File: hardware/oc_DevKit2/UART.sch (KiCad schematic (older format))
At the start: 6 parts, among them U1 CP2102N

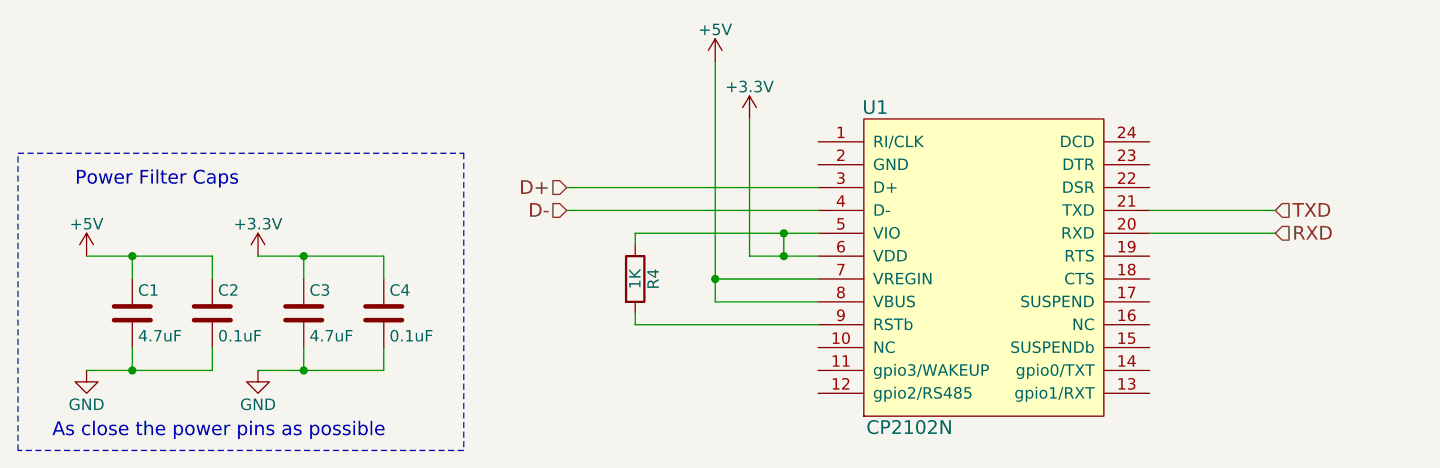
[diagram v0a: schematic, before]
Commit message: Lil Patch
Small changes. Updating for forthcoming Lite branch updates
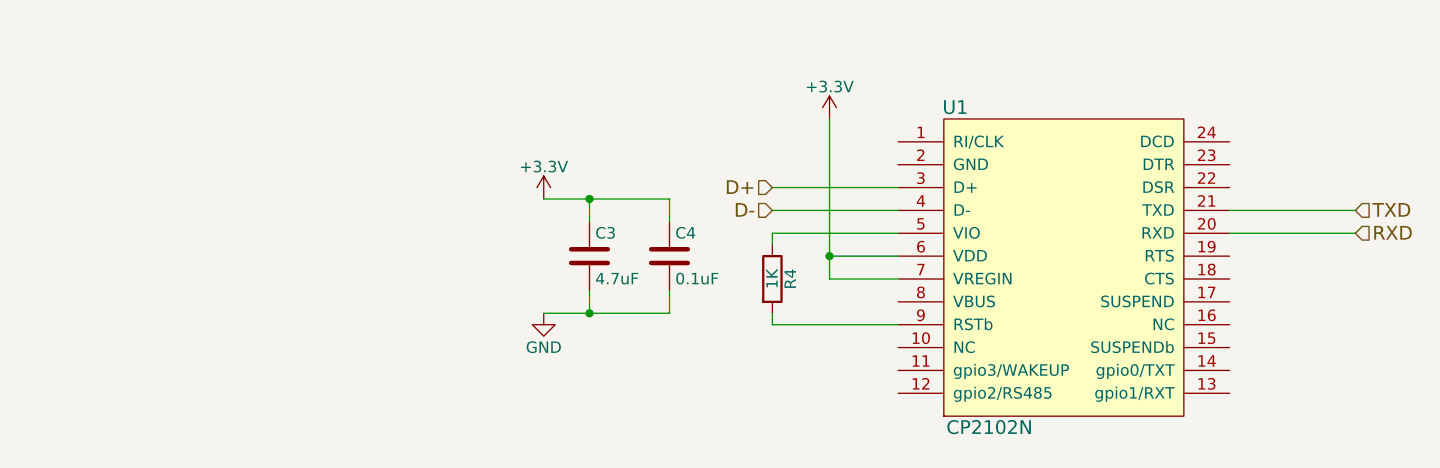
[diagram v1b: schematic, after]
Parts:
- removed C1: 4.7uF, Capacitors_SMD:C_0805_HandSoldering, symbol C
- removed C2: 0.1uF, Capacitors_SMD:C_0805_HandSoldering, symbol C
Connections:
- net +3V3: now also U1.7 (VREGIN); no longer R4.1, U1.5 (VIO)
- net +5V: no longer names the net of U1.8 (VBUS)
- net +5V: no longer U1.7 (VREGIN)
- new net: R4.1, U1.5 (VIO)
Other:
- note removed: "As close the power pins as possible"
- note removed: "Power Filter Caps"
- moved on the sheet: C3, C4, R4, U1
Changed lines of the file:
@@
 L CP2102N U1
 U 1 1 59C93D7F
-P 5850 4600
-F 0 "U1" H 5350 5950 60  0000 C CNN
-F 1 "CP2102N" H 5500 4550 60  0000 C CNN
-F 2 "Housings_DFN_QFN:QFN-24_4x4mm_Pitch0.5mm" H 5700 4600 60  0001 C CNN
-F 3 "" H 5700 4600 60  0001 C CNN
-	1    5850 4600
+P 6200 4600
+F 0 "U1" H 5700 5950 60  0000 C CNN
+F 1 "CP2102N" H 5850 4550 60  0000 C CNN
+F 2 "Housings_DFN_QFN:QFN-24_4x4mm_Pitch0.5mm" H 6050 4600 60  0001 C CNN
+F 3 "" H 6050 4600 60  0001 C CNN
+	1    6200 4600
 	1    0    0    -1
 $EndComp
@@
 L R R4
 U 1 1 59C9487D
-P 4300 4000
-F 0 "R4" V 4380 4000 50  0000 C CNN
-F 1 "1K" V 4300 4000 50  0000 C CNN
-F 2 "Resistors_SMD:R_0805_HandSoldering" V 4230 4000 50  0001 C CNN
-F 3 "" H 4300 4000 50  0001 C CNN
-	1    4300 4000
+P 4900 4000
+F 0 "R4" V 4980 4000 50  0000 C CNN
+F 1 "1K" V 4900 4000 50  0000 C CNN
+F 2 "Resistors_SMD:R_0805_HandSoldering" V 4830 4000 50  0001 C CNN
+F 3 "" H 4900 4000 50  0001 C CNN
+	1    4900 4000
 	1    0    0    -1
 $EndComp
@@
 L C C3
 U 1 1 59C94915
-P 2850 4150
-F 0 "C3" H 2875 4250 50  0000 L CNN
-F 1 "4.7uF" H 2875 4050 50  0000 L CNN
-F 2 "Capacitors_SMD:C_0805_HandSoldering" H 2888 4000 50  0001 C CNN
-F 3 "" H 2850 4150 50  0001 C CNN
-	1    2850 4150
-	1    0    0    -1
-$EndComp
-$Comp
-L C C1
-U 1 1 59C94A49
-P 2100 4150
-F 0 "C1" H 2125 4250 50  0000 L CNN
-F 1 "4.7uF" H 2125 4050 50  0000 L CNN
-F 2 "Capacitors_SMD:C_0805_HandSoldering" H 2138 4000 50  0001 C CNN
-F 3 "" H 2100 4150 50  0001 C CNN
-	1    2100 4150
-	1    0    0    -1
-$EndComp
-$Comp
-L C C2
-U 1 1 59C94A6F
-P 2450 4150
-F 0 "C2" H 2475 4250 50  0000 L CNN
-F 1 "0.1uF" H 2475 4050 50  0000 L CNN
-F 2 "Capacitors_SMD:C_0805_HandSoldering" H 2488 4000 50  0001 C CNN
-F 3 "" H 2450 4150 50  0001 C CNN
-	1    2450 4150
+P 4100 3900
+F 0 "C3" H 4125 4000 50  0000 L CNN
+F 1 "4.7uF" H 4125 3800 50  0000 L CNN
+F 2 "Capacitors_SMD:C_0805_HandSoldering" H 4138 3750 50  0001 C CNN
+F 3 "" H 4100 3900 50  0001 C CNN
+	1    4100 3900
 	1    0    0    -1
 $EndComp
@@
 L C C4
 U 1 1 59C94ADB
-P 3200 4150
-F 0 "C4" H 3225 4250 50  0000 L CNN
-F 1 "0.1uF" H 3225 4050 50  0000 L CNN
-F 2 "Capacitors_SMD:C_0805_HandSoldering" H 3238 4000 50  0001 C CNN
-F 3 "" H 3200 4150 50  0001 C CNN
-	1    3200 4150
+P 4450 3900
+F 0 "C4" H 4475 4000 50  0000 L CNN
+F 1 "0.1uF" H 4475 3800 50  0000 L CNN
+F 2 "Capacitors_SMD:C_0805_HandSoldering" H 4488 3750 50  0001 C CNN
+F 3 "" H 4450 3900 50  0001 C CNN
+	1    4450 3900
 	1    0    0    -1
 $EndComp
@@
 L GND #PWR017
 U 1 1 59C94DA8
-P 2650 4400
-F 0 "#PWR017" H 2650 4150 50  0001 C CNN
-F 1 "GND" H 2650 4250 50  0000 C CNN
-F 2 "" H 2650 4400 50  0001 C CNN
-F 3 "" H 2650 4400 50  0001 C CNN
-	1    2650 4400
+P 3900 4150
+F 0 "#PWR017" H 3900 3900 50  0001 C CNN
+F 1 "GND" H 3900 4000 50  0000 C CNN
+F 2 "" H 3900 4150 50  0001 C CNN
+F 3 "" H 3900 4150 50  0001 C CNN
+	1    3900 4150
 	1    0    0    -1
 $EndComp
 $Comp
-L GND #PWR018
-U 1 1 59C94DCF
-P 1900 4400
-F 0 "#PWR018" H 1900 4150 50  0001 C CNN
-F 1 "GND" H 1900 4250 50  0000 C CNN
-F 2 "" H 1900 4400 50  0001 C CNN
-F 3 "" H 1900 4400 50  0001 C CNN
-	1    1900 4400
+L +3.3V #PWR018
+U 1 1 59C94E0C
+P 3900 3650
+F 0 "#PWR018" H 3900 3500 50  0001 C CNN
+F 1 "+3.3V" H 3900 3790 50  0000 C CNN
+F 2 "" H 3900 3650 50  0001 C CNN
+F 3 "" H 3900 3650 50  0001 C CNN
+	1    3900 3650
 	1    0    0    -1
 $EndComp
 $Comp
-L +5V #PWR019
-U 1 1 59C94DEA
-P 1900 3900
-F 0 "#PWR019" H 1900 3750 50  0001 C CNN
-F 1 "+5V" H 1900 4040 50  0000 C CNN
-F 2 "" H 1900 3900 50  0001 C CNN
-F 3 "" H 1900 3900 50  0001 C CNN
-	1    1900 3900
-	1    0    0    -1
-$EndComp
-$Comp
-L +3.3V #PWR020
-U 1 1 59C94E0C
-P 2650 3900
-F 0 "#PWR020" H 2650 3750 50  0001 C CNN
-F 1 "+3.3V" H 2650 4040 50  0000 C CNN
-F 2 "" H 2650 3900 50  0001 C CNN
-F 3 "" H 2650 3900 50  0001 C CNN
-	1    2650 3900
-	1    0    0    -1
-$EndComp
-$Comp
-L +3.3V #PWR021
+L +3.3V #PWR019
 U 1 1 59C94E58
-P 4800 3300
-F 0 "#PWR021" H 4800 3150 50  0001 C CNN
-F 1 "+3.3V" H 4800 3440 50  0000 C CNN
-F 2 "" H 4800 3300 50  0001 C CNN
-F 3 "" H 4800 3300 50  0001 C CNN
-	1    4800 3300
-	1    0    0    -1
-$EndComp
-$Comp
-L +5V #PWR022
-U 1 1 59C94E99
-P 4650 3050
-F 0 "#PWR022" H 4650 2900 50  0001 C CNN
-F 1 "+5V" H 4650 3190 50  0000 C CNN
-F 2 "" H 4650 3050 50  0001 C CNN
-F 3 "" H 4650 3050 50  0001 C CNN
-	1    4650 3050
+P 5150 3300
+F 0 "#PWR019" H 5150 3150 50  0001 C CNN
+F 1 "+3.3V" H 5150 3440 50  0000 C CNN
+F 2 "" H 5150 3300 50  0001 C CNN
+F 3 "" H 5150 3300 50  0001 C CNN
+	1    5150 3300
 	1    0    0    -1
 $EndComp
 Wire Wire Line
-	5100 3800 4300 3800
+	5450 3800 4900 3800
 Wire Wire Line
-	4300 3800 4300 3850
+	4900 3800 4900 3850
 Wire Wire Line
-	4300 4150 4300 4200
+	4900 4150 4900 4200
 Wire Wire Line
-	4300 4200 5100 4200
+	4900 4200 5450 4200
 Wire Wire Line
-	1900 3900 2450 3900
+	3900 3650 4450 3650
 Wire Wire Line
-	2450 3900 2450 4000
+	4450 3650 4450 3750
 Wire Wire Line
-	2100 4000 2100 3900
-Connection ~ 2100 3900
+	3900 4150 4450 4150
 Wire Wire Line
-	2450 4400 2450 4300
+	4450 4150 4450 4050
 Wire Wire Line
-	1900 4400 2450 4400
+	4100 4150 4100 4050
+Connection ~ 4100 4150
 Wire Wire Line
-	2100 4300 2100 4400
-Connection ~ 2100 4400
+	4100 3750 4100 3650
+Connection ~ 4100 3650
 Wire Wire Line
-	2650 3900 3200 3900
+	5150 3300 5150 4000
 Wire Wire Line
-	3200 3900 3200 4000
+	5150 4000 5450 4000
 Wire Wire Line
-	2650 4400 3200 4400
+	5150 3900 5450 3900
 Wire Wire Line
-	3200 4400 3200 4300
+	4900 3600 5450 3600
 Wire Wire Line
-	2850 4400 2850 4300
-Connection ~ 2850 4400
+	4900 3700 5450 3700
 Wire Wire Line
-	2850 4000 2850 3900
-Connection ~ 2850 3900
+	6900 3700 7450 3700
 Wire Wire Line
-	4800 3900 4800 3300
-Wire Wire Line
-	4650 3050 4650 4100
-Wire Wire Line
-	4650 4000 5100 4000
-Wire Wire Line
-	4800 3900 5100 3900
-Wire Wire Line
-	4650 4100 5100 4100
-Wire Wire Line
-	4000 3600 5100 3600
-Wire Wire Line
-	4000 3700 5100 3700
-Wire Wire Line
-	6550 3700 7100 3700
-Wire Wire Line
-	6550 3800 7100 3800
-Text HLabel 7100 3700 2    60   Input ~ 0
+	6900 3800 7450 3800
+Text HLabel 7450 3700 2    60   Input ~ 0
 TXD
-Text HLabel 7100 3800 2    60   Input ~ 0
+Text HLabel 7450 3800 2    60   Input ~ 0
 RXD
-Connection ~ 4650 4000
-Text HLabel 4000 3600 0    60   Input ~ 0
+Text HLabel 4900 3600 0    60   Input ~ 0
 D+
-Text HLabel 4000 3700 0    60   Input ~ 0
+Text HLabel 4900 3700 0    60   Input ~ 0
 D-
-Text Notes 1750 4700 0    60   ~ 0
-As close the power pins as possible
-Text Notes 1850 3600 0    60   ~ 0
-Power Filter Caps
-Wire Notes Line
-	1600 3450 3550 3450
-Wire Notes Line
-	3550 3450 3550 4750
-Wire Notes Line
-	3550 4750 1600 4750
-Wire Notes Line
-	1600 4750 1600 3450
-Wire Wire Line
-	4950 3800 4950 3900
-Connection ~ 4950 3900
-Connection ~ 4950 3800
+Connection ~ 5150 3900
 $EndSCHEMATC
